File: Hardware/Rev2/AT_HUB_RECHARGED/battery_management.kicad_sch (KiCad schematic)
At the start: 39 parts, among them J13 Pack Thermister, J14 Through Hole, J15 EXT Charge Port, J16 USB_C_Receptacle_PowerOnly_6P, J2 JST, Q1 NTR1P02T1G, Q2 NTR1P02T1G, SW11 SW_SPDT, U7 BQ21040DBV, U8 TLV61070ADBV, U9 BQ27427YZFR

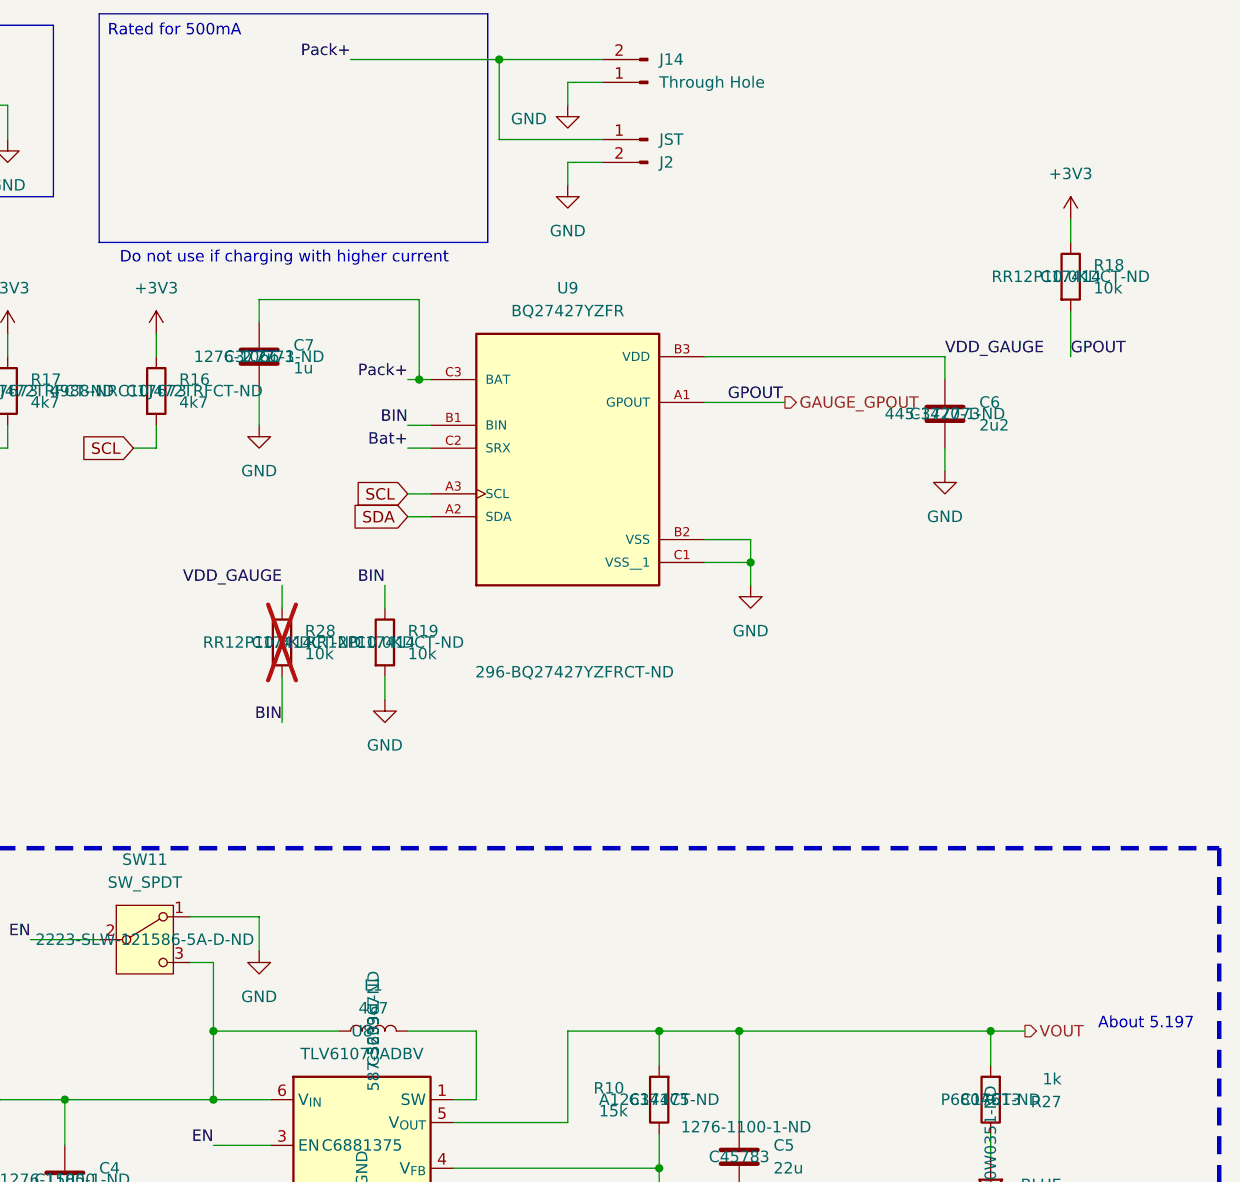
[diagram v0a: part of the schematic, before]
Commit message: Done the design will verify
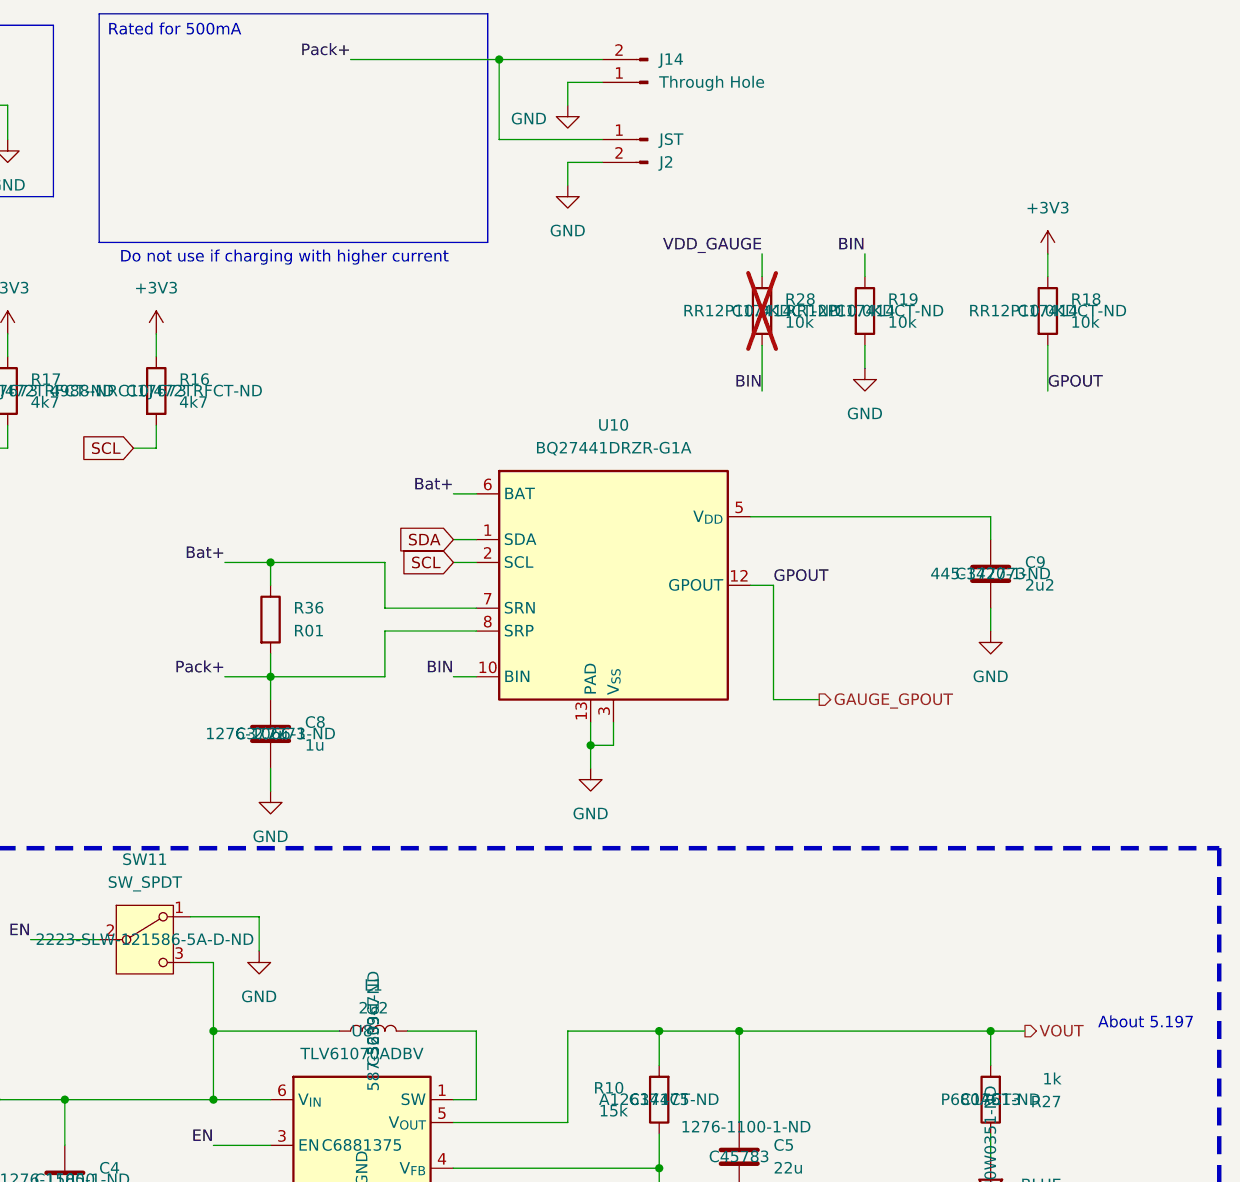
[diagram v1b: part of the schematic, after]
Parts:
- removed C6: 2u2, Capacitor_SMD:C_0805_2012Metric, symbol Device:C
- removed C7: 1u, Capacitor_SMD:C_0805_2012Metric, symbol Device:C
- removed U9: BQ27427YZFR, AT_HUB_R2:IC_BQ27427YZFR, symbol AT_HUB_R2:BQ27427YZFR
- added C8: 1u, Capacitor_SMD:C_0805_2012Metric, symbol Device:C
- added C9: 2u2, Capacitor_SMD:C_0805_2012Metric, symbol Device:C
- added R36: R01, Resistor_SMD:R_0805_2012Metric, symbol Device:R
- added U10: BQ27441DRZR-G1A, Package_SON:Texas_S-PDSO-N12, symbol Battery_Management:BQ27441DRZR-G1A
- L1: value 4u7 -> 2u2
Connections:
- net BIN: now also U10.10 (BIN)
- net Bat+: now also R36.1, U10.6 (BAT), U10.7 (SRN)
- net GAUGE_GPOUT: now also U10.12 (GPOUT)
- net GND: now also C8.2, C9.2, U10.13 (PAD), U10.3 (V_{SS})
- net Pack+: now also C8.1, R36.2, U10.8 (SRP)
- net SCL: now also U10.2 (SCL)
- net SDA: now also U10.1 (SDA)
- new net: C9.1, U10.5 (V_{DD})
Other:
- moved on the sheet: R18, R19, R28

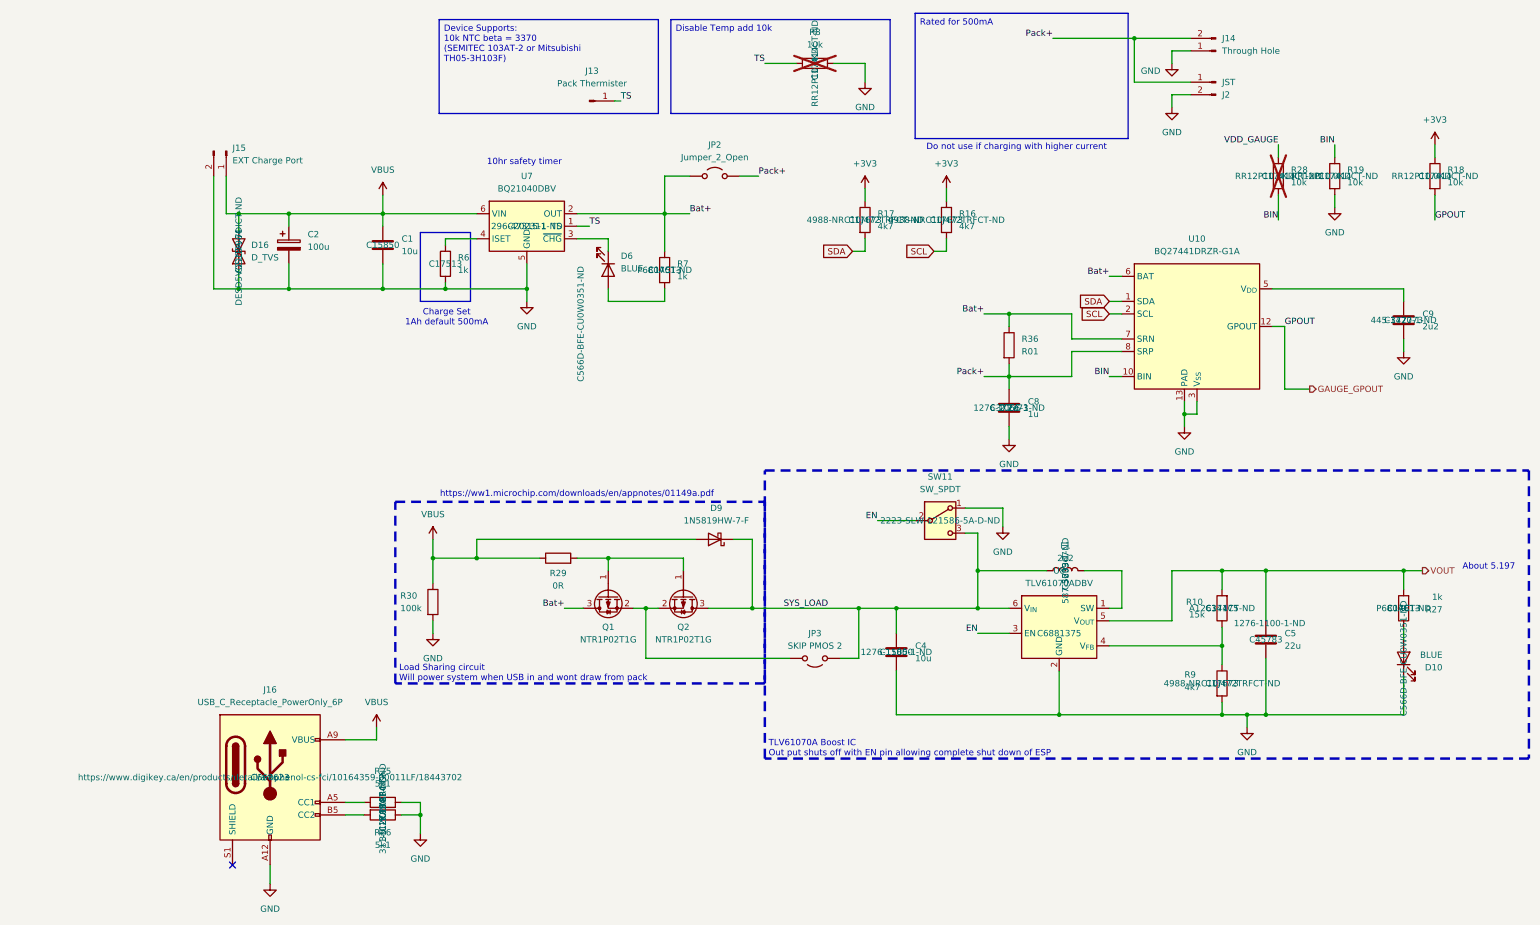
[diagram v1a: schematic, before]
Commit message: Added Rev 3
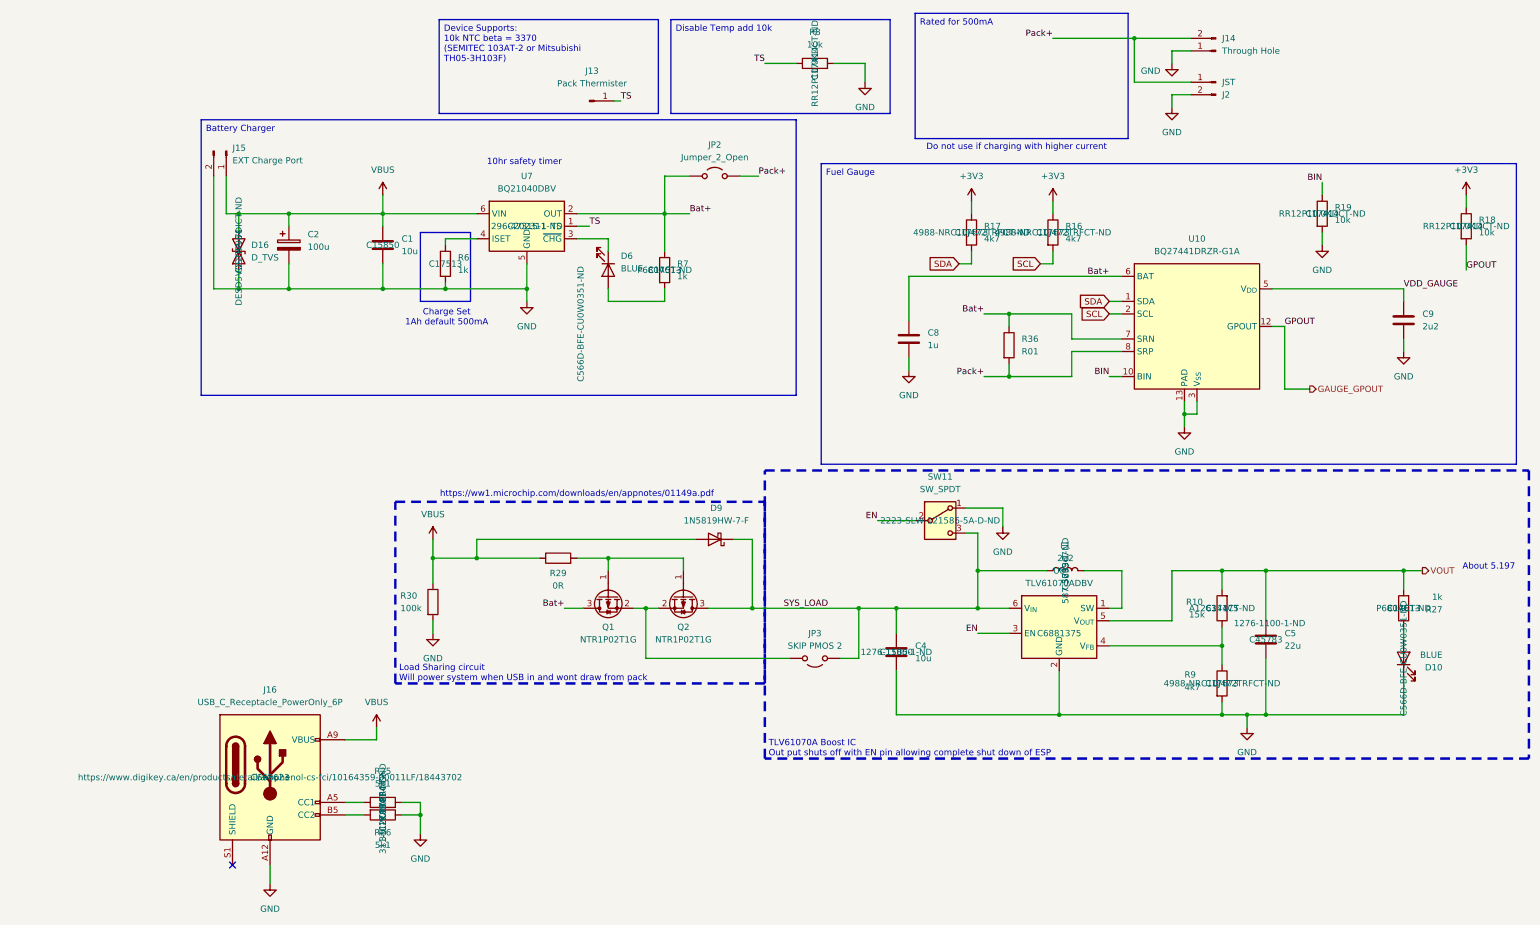
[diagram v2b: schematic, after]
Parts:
- removed R28: 10k, Resistor_SMD:R_0805_2012Metric, symbol Device:R
- C2: footprint Capacitor_SMD:C_Elec_6.3x7.7 -> Capacitor_Tantalum_SMD:CP_EIA-3216-18_Kemet-A
- R8: now fitted
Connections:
- net Bat+: now also C8.1
- net Pack+: no longer C8.1
- net VDD_GAUGE: now also C9.1, U10.5 (V_{DD})
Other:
- moved on the sheet: C8, R16, R17, R18, R19
